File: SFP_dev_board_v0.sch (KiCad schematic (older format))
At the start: 47 parts, among them J1 Conn_02x01_Row_Letter_First, J2 Conn_02x01_Row_Letter_First, P1 CONN_02X10, P2 SFP CAGE, SW1 SW_Push_Dual, SW2 SW_Push_Dual, SW3 SW_Push_Dual, SW4 SW_Push_Dual, U1 LD1117AV33, U2 SN65EPT22, U3 SN65LVELT23

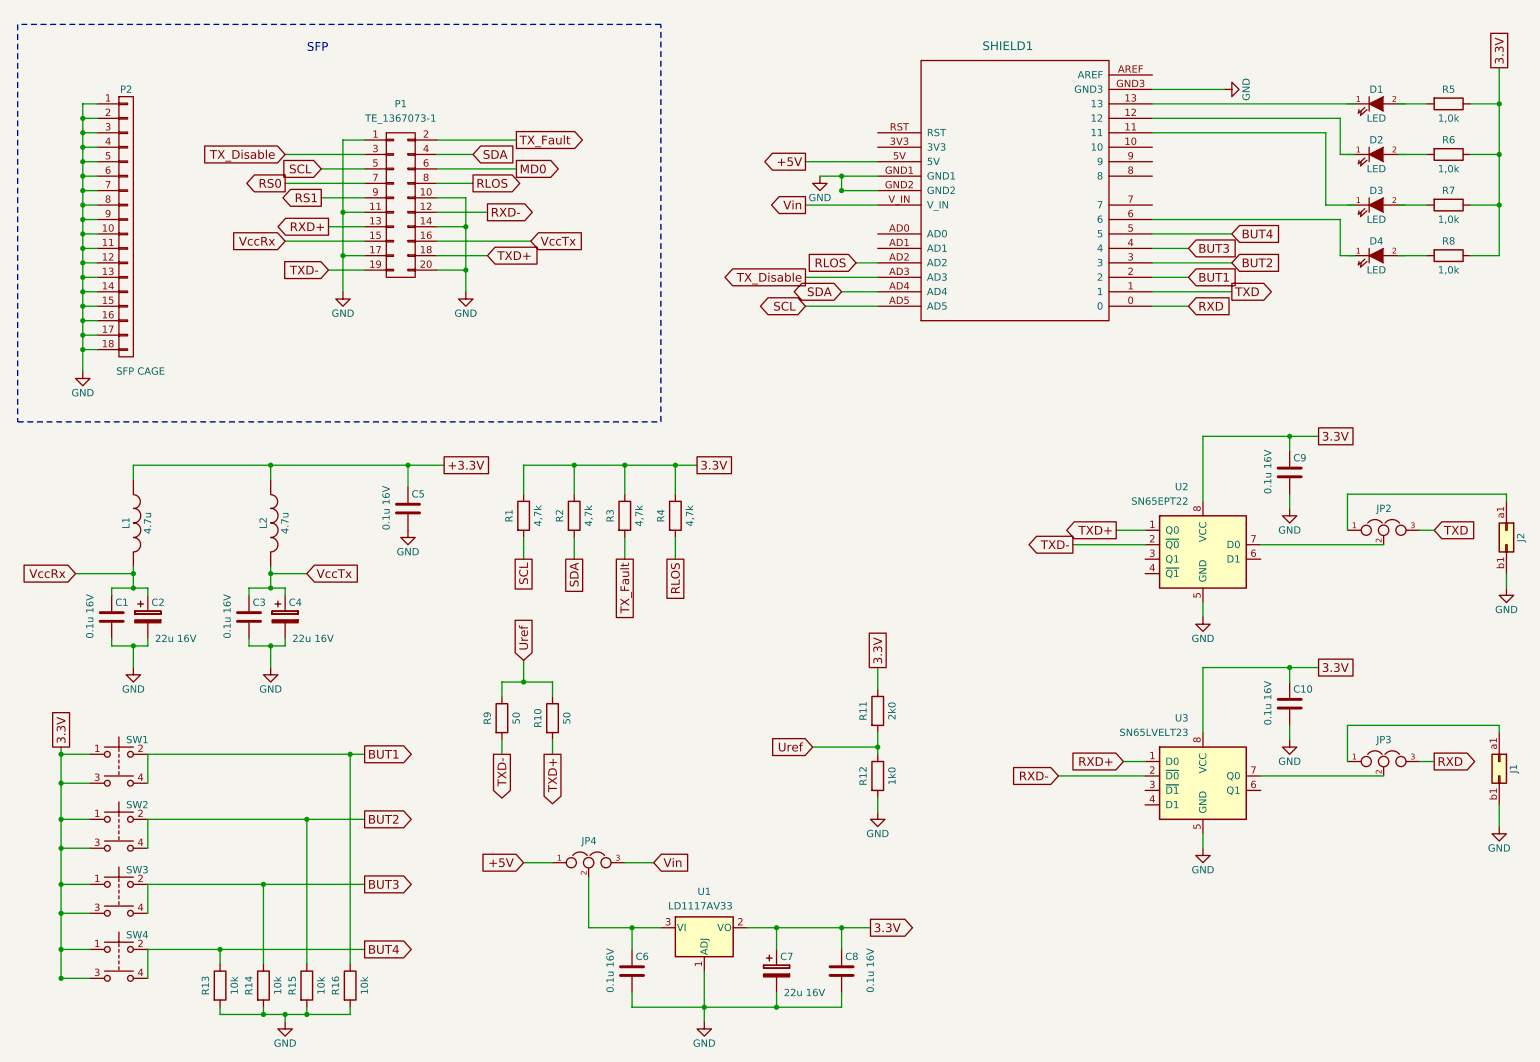
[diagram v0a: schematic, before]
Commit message: buffers
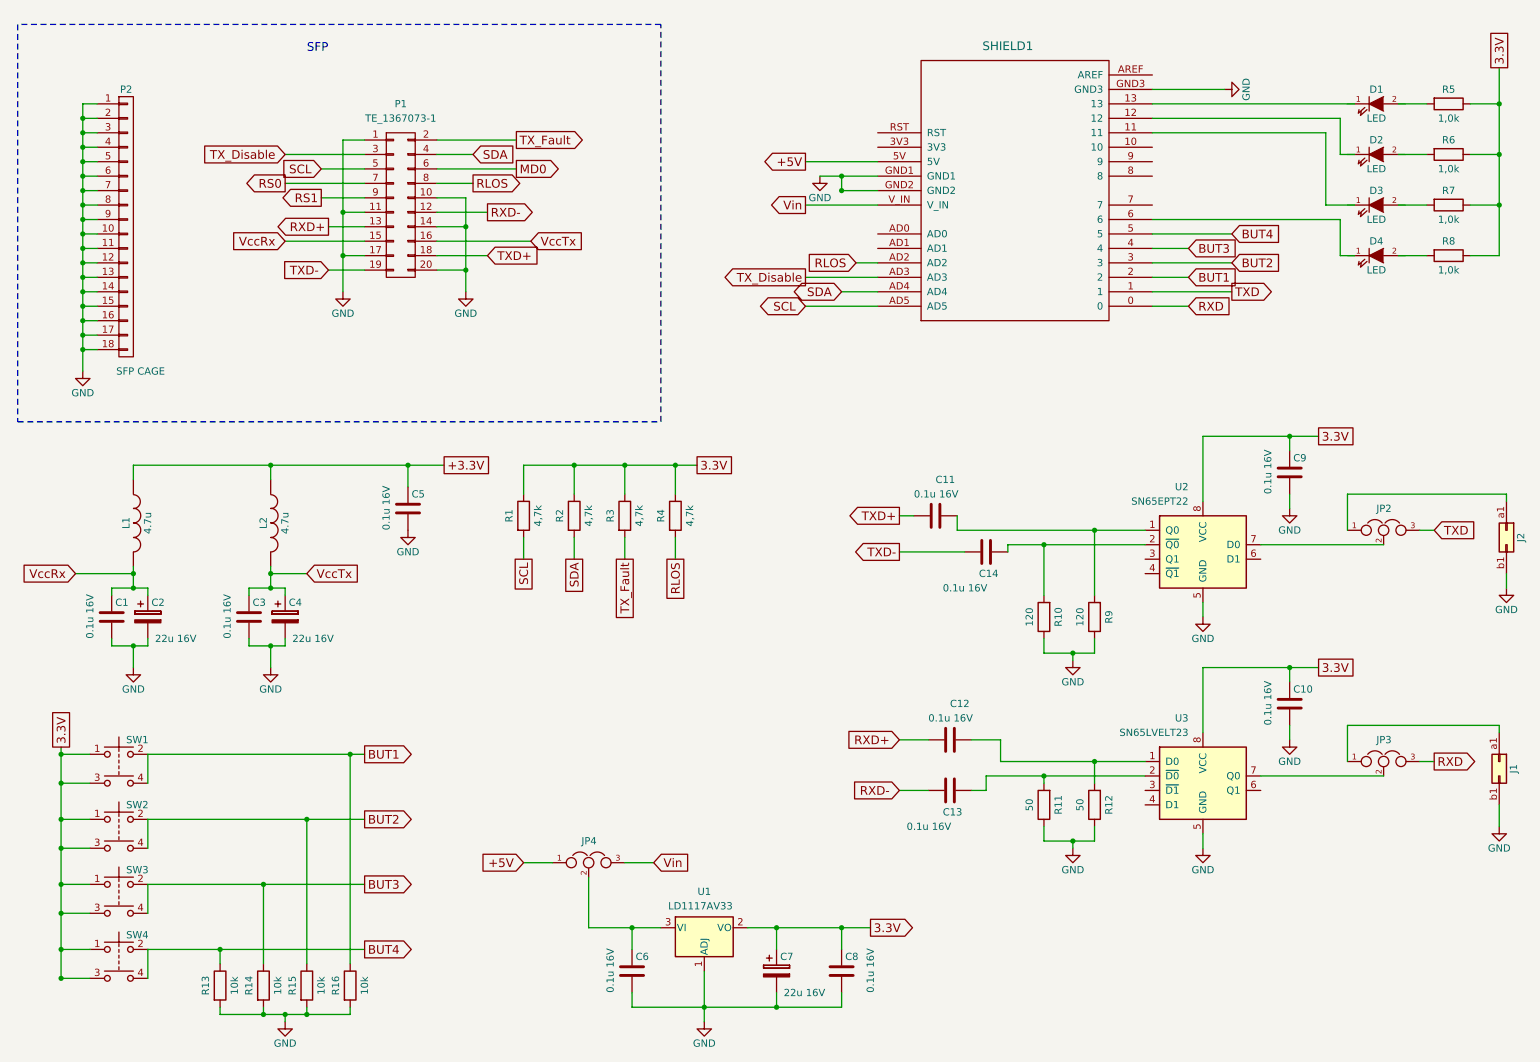
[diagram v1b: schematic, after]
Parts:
- added C11, C12, C13, C14: 0.1u 16V, Capacitors_SMD:C_0805_HandSoldering, symbol C
- R10, R9: value 50 -> 120
- R11: value 2k0 -> 50
- R12: value 1k0 -> 50
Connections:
- net labels removed: Uref
- wire segments 183 -> 195
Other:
- moved on the sheet: R10, R9
